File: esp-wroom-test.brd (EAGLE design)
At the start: 35.7 x 27.4 mm, 15 parts, among them U8 NCP1117LPST50T3G

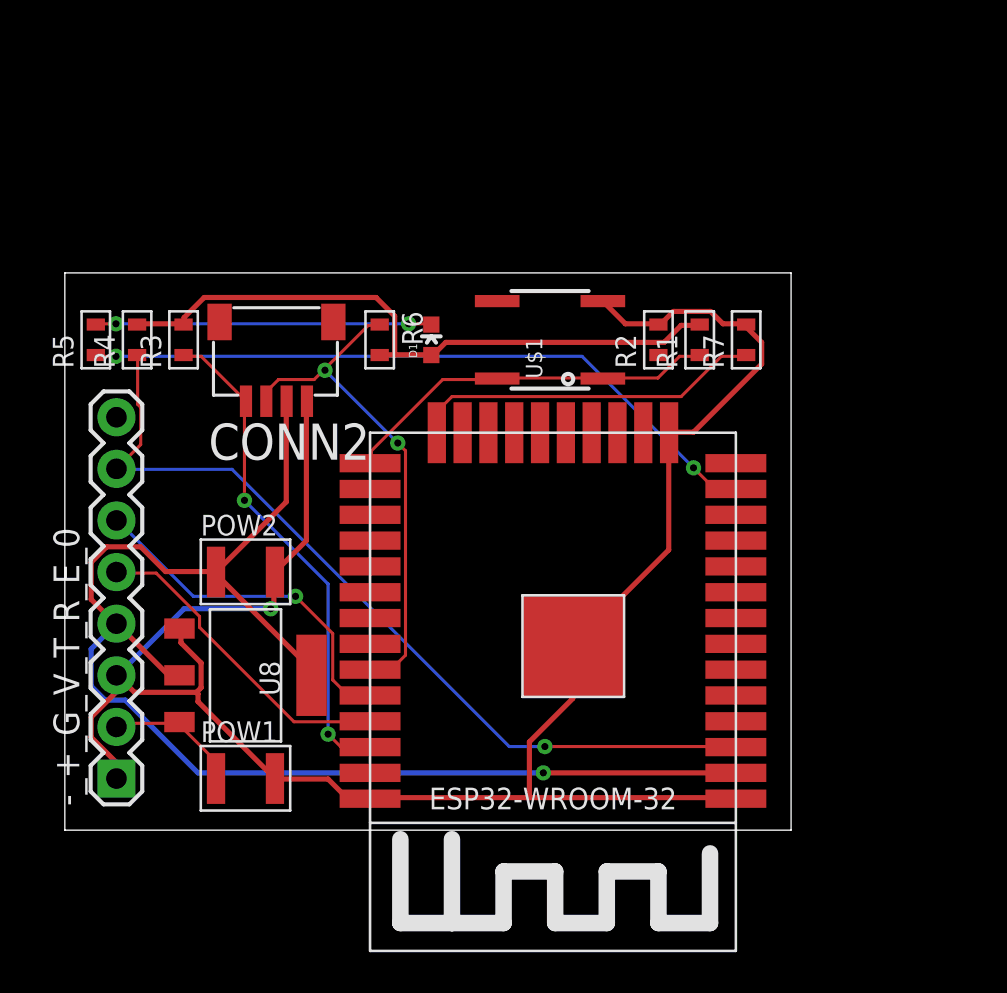
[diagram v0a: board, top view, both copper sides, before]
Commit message: as ordered
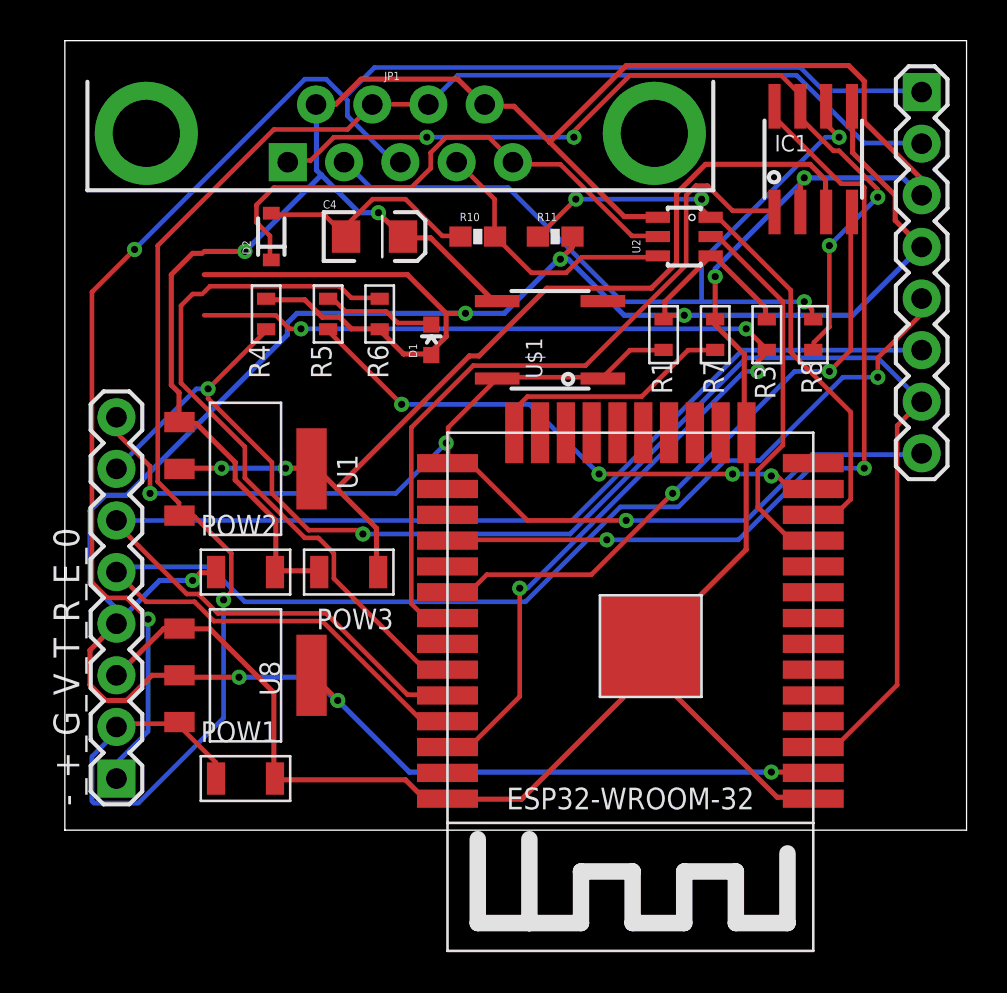
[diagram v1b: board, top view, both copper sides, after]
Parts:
- removed CONN2: STEMMA_I2C_QT, 00jim:JST_SH4
- removed R2: (no value), 00jim:R0603
- added -_+_G_V_T_R_E_1: MF-CON-2.54mm-01x08, SparkFun-Connectors:1X08
- added C4: 10uF, SparkFun-Capacitors:EIA3216
- added D2: BAS16, SparkFun-DiscreteSemi:SOD-323
- added IC1: TCAN1051HGV, microbuilder:SOIC8_150MIL
- added JP1: DB9, SparkFun-Connectors:DB9
- added POW3: (no value), MF_Passives:C1206
- added R10, R11: 10K, SparkFun-Resistors:0603-RES
- added R8: 200, 00jim:R0603
- added U1: NCP1117LPST50T3G, MF_IC_Power:SOT-223-3
- added U2: XN04312, SparkFun-DiscreteSemi:SOT23-6
- POW1, POW2: device MF_Passives:C1210 -> MF_Passives:C1206
- moved R3 28.7 mm to (34.5, 24.4)
- moved R5 11.5 mm to (13.0, 25.4)
- moved R4 6.48 mm to (9.91, 25.4)
- moved U$3 3.81 mm to (36.8, 19.6)
- moved R1 1.80 mm to (29.5, 24.4)
- moved R7 1.55 mm to (32.0, 24.4)
- moved R6 1.27 mm to (15.5, 25.4)
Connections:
- removed net IO0: -_+_G_V_T_R_E_0.8
- removed net IO12: U$3.IO12
- removed net IO15: U$3.IO15
- removed net PD: R2.P$1
- removed net VCC1: D1.A, R1.P$2, R3.P$2, R4.P$2, R6.P$2
- new net CANRX: IC1.4, U$3.IO18
- new net CANTX: IC1.1, U$3.IO19
- new net CAN_H: IC1.7, JP1.1, R8.P$1
- new net CAN_L: IC1.6, JP1.2, R8.P$2
- new net CAN_S: IC1.8, U$3.IO17
- new net DB9_RX: U$3.IO26, U2.2
- new net DB9_TX: R11.1, U$3.IO27, U2.1
- new net N$4: C4.C, D2.A, R10.1
- new net RS-IN: D2.C, JP1.5, U2.5
- new net RS-OUT: JP1.4, R10.2, U2.4
- new net UNITID: -_+_G_V_T_R_E_0.1, -_+_G_V_T_R_E_1.1, JP1.3
- new net VCC_50: IC1.3, POW3.P$1, U1.P$1, U1.P$3
- net EN: now also -_+_G_V_T_R_E_1.7
- net GND: now also -_+_G_V_T_R_E_1.3, C4.A, IC1.2, JP1.6, JP1.9, POW3.P$2, U1.P$2, U2.6; no longer -_+_G_V_T_R_E_0.1, CONN2.1, R2.P$2
- net IO00: now also -_+_G_V_T_R_E_0.8, -_+_G_V_T_R_E_1.8
- net RAW: now also -_+_G_V_T_R_E_1.2, JP1.7, JP1.8, U1.P$4
- net RXI: now also -_+_G_V_T_R_E_1.6
- net SCL: no longer CONN2.4
- net SDA: no longer CONN2.3
- net TXO: now also -_+_G_V_T_R_E_1.5
- net VCC: now also -_+_G_V_T_R_E_1.4, D1.A, IC1.5, R1.P$2, R11.2, R3.P$2, R4.P$2, R6.P$2, U2.3; no longer CONN2.2
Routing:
- net VCC: track 68.6 -> 149.8 mm, vias 1 -> 7
- net RAW: track 6.76 -> 86.9 mm, vias 0 -> 1
- net UNITID: track 0.00 -> 77.5 mm, vias 0 -> 2
- net GND: track 100.4 -> 172.0 mm, vias 1 -> 4
- net TXO: track 15.9 -> 67.0 mm, vias 0 -> 1
- net VCC_50: track 0.00 -> 47.7 mm, vias 0 -> 2
- net RXI: track 17.4 -> 63.1 mm, vias 1 -> 0
- net CAN_H: track 0.00 -> 43.2 mm, vias 0 -> 4
- net CAN_S: track 0.00 -> 42.2 mm, vias 0 -> 2
- net IO00: track 18.8 -> 60.0 mm, vias 0 -> 3
- net CAN_L: track 0.00 -> 39.6 mm, vias 0 -> 2
- net CANTX: track 0.00 -> 36.1 mm
- net VCC1: track 32.1 -> 0.00 mm
- net CANRX: track 0.00 -> 31.6 mm, vias 0 -> 2
- net EN: track 42.3 -> 73.8 mm, vias 1 -> 2
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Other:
- board size 35.7 x 27.4 mm -> 44.4 x 38.9 mm
